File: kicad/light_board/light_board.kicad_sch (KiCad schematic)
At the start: 16 parts

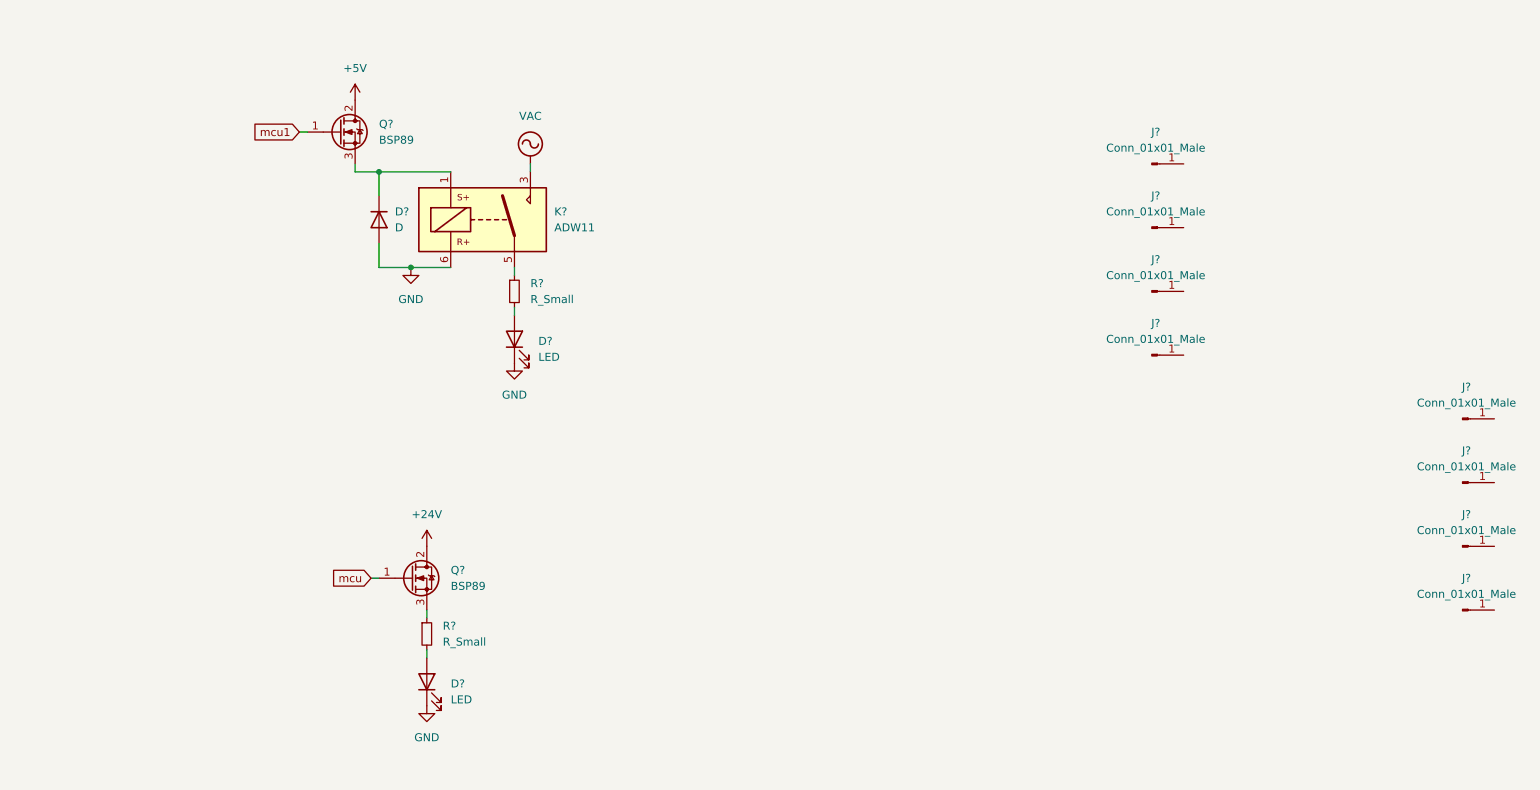
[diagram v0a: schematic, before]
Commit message: traffic lights WIP
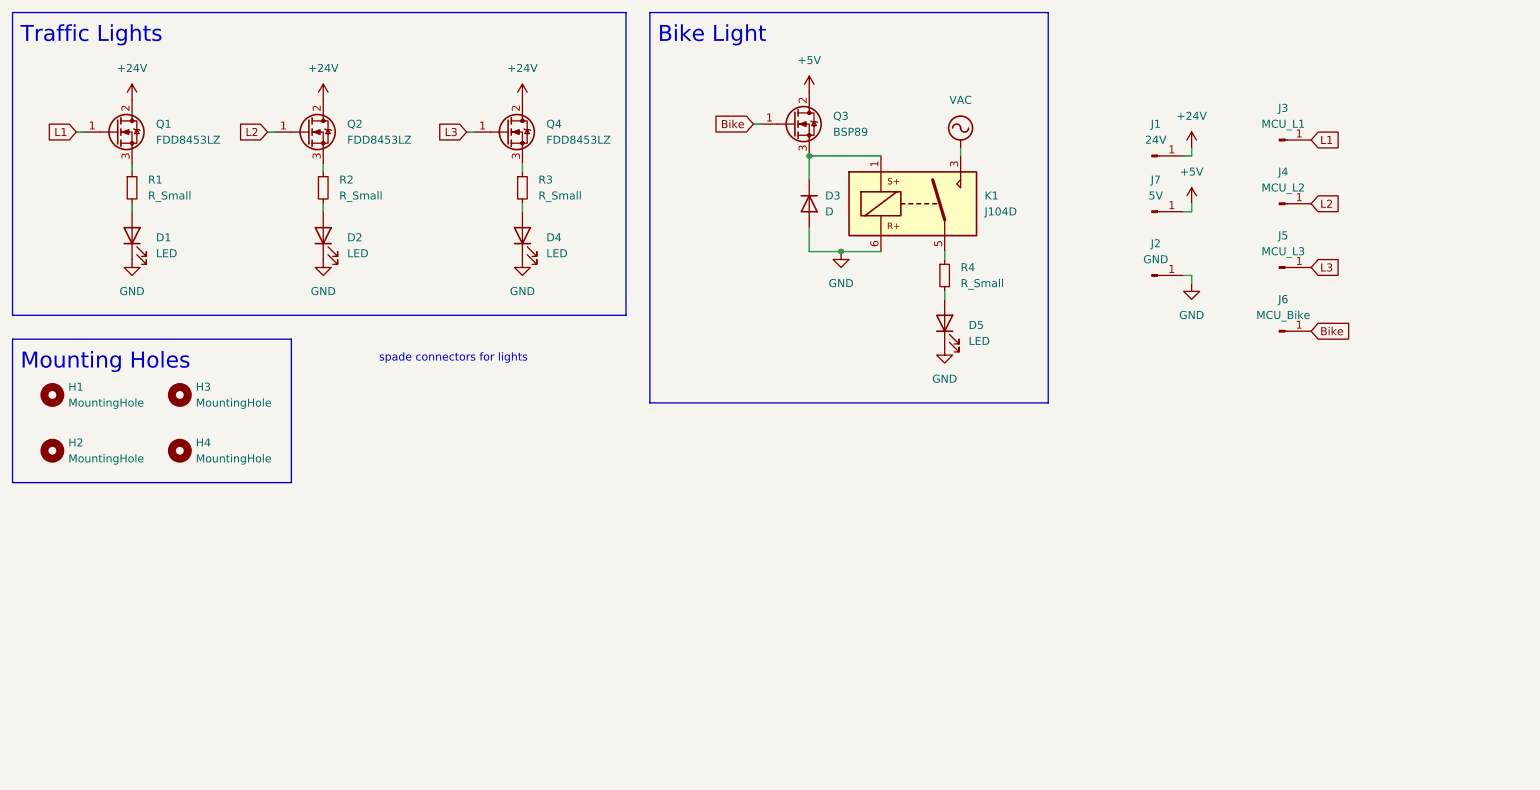
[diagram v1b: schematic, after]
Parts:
- removed J? (x3): Conn_01x01_Male, symbol Connector:Conn_01x01_Male
- added D2, D4: LED, symbol Device:LED
- added H1, H2, H3, H4: MountingHole, symbol Mechanical:MountingHole
- added J6: MCU_Bike, symbol Connector:Conn_01x01_Male
- added J7: 5V, symbol Connector:Conn_01x01_Male
- added Q2, Q4: FDD8453LZ, Package_TO_SOT_SMD:SOT-223-3_TabPin2, symbol Transistor_FET:BSP89
- added R2, R3: R_Small, symbol Device:R_Small
- J1: renamed from J?; value Conn_01x01_Male -> 24V
- J2: renamed from J?; value Conn_01x01_Male -> GND
- J3: renamed from J?; value Conn_01x01_Male -> MCU_L1
- J4: renamed from J?; value Conn_01x01_Male -> MCU_L2
- J5: renamed from J?; value Conn_01x01_Male -> MCU_L3
- K1: renamed from K?; value ADW11 -> J104D
- Q1: renamed from Q?; value BSP89 -> FDD8453LZ
- gave numbers to parts that had none: 6
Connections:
- net mcu is gone; now on net L1: Q1.1 (G)
- net +24V: now also J1.1 (Pin_1), Q2.2 (D), Q4.2 (D)
- net +5V: now also J7.1 (Pin_1)
- net GND: now also J2.1 (Pin_1), D2.1 (K), D4.1 (K)
- net L1: now reaches J3.1 (Pin_1)
- net L2: now reaches J4.1 (Pin_1)
- net L2: now also Q2.1 (G)
- net L3: now reaches J5.1 (Pin_1)
- net L3: now also Q4.1 (G)
- net mcu1 renamed Bike
- net Bike: now also J6.1 (Pin_1)
- new net: Q2.3 (S), R2.1
- new net: D4.2 (A), R3.2
- new net: Q4.3 (S), R3.1
- new net: D2.2 (A), R2.2
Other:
- note added: "Bike Light"
- note added: "Mounting Holes"
- note added: "Traffic Lights"
- note added: "spade connectors for lights"
- moved on the sheet: D1, D3, D5, J1, J2, J3, J4, J5, K1, Q1, Q3, R1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

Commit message: light board done
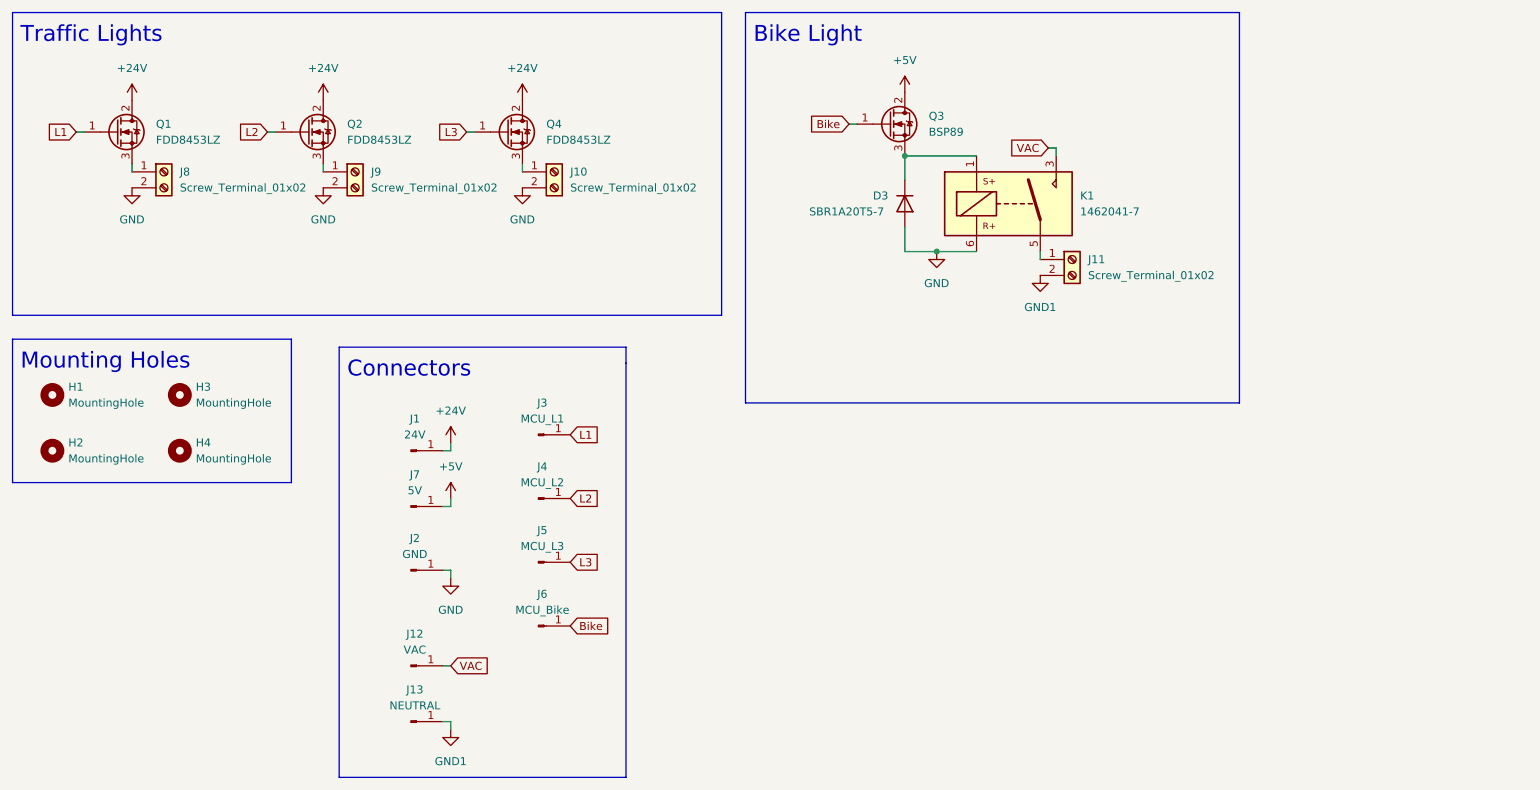
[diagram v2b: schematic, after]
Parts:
- removed D1, D2, D4, D5: LED, symbol Device:LED
- removed R1, R2, R3, R4: R_Small, symbol Device:R_Small
- added J10, J11, J8, J9: Screw_Terminal_01x02, TerminalBlock:TerminalBlock_Altech_AK300-2_P5.00mm, symbol Connector:Screw_Terminal_01x02
- added J12: VAC, Connector_PinHeader_2.54mm:PinHeader_1x01_P2.54mm_Vertical, symbol Connector:Conn_01x01_Male
- added J13: NEUTRAL, Connector_PinHeader_2.54mm:PinHeader_1x01_P2.54mm_Vertical, symbol Connector:Conn_01x01_Male
- D3: value D -> SBR1A20T5-7; footprint (none) -> Diode_SMD:D_SOD-523
- H1, H2, H3, H4: footprint (none) -> MountingHole:MountingHole_3.5mm
- J1, J2, J3, J4, J5, J6, J7: footprint (none) -> Connector_PinHeader_2.54mm:PinHeader_1x01_P2.54mm_Vertical
- K1: value J104D -> 1462041-7; footprint Relay_THT:Relay_1P1T_NO_10x24x18.8mm_Panasonic_ADW11xxxxW_THT -> _mine:1462041-7
- Q1, Q2, Q3, Q4: footprint Package_TO_SOT_SMD:SOT-223-3_TabPin2 -> Package_TO_SOT_SMD:TO-252-2
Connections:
- net GND: now also J10.2 (Pin_2), J8.2 (Pin_2), J9.2 (Pin_2)
- net VAC: now also J12.1 (Pin_1)
- net at Q2.3 (S): now also J9.1 (Pin_1)
- net at Q4.3 (S): now also J10.1 (Pin_1)
- net at Q1.3 (S): now also J8.1 (Pin_1)
- net at K1.5: now also J11.1 (Pin_1)
- new net GND1: J11.2 (Pin_2), J13.1 (Pin_1)
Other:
- note added: "Connectors"
- note removed: "spade connectors for lights"
- moved on the sheet: D3, J1, J2, J3, J4, J5, J6, J7, K1, Q3
